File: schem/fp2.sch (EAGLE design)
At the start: 24 parts, among them IC1 74HC377N, IC10 74HC377N, IC11 74HC08N, IC12 ULN2003AN, IC13 ULN2003AN, IC14 ULN2003AN, IC15 74HC14N, IC2 74HC244N, IC3 74HC377N, IC4 74HC244N, IC5 74HC244N, IC6 74HC244N, IC7 74HC32N, IC8 74HC244N, IC9 74HC244N

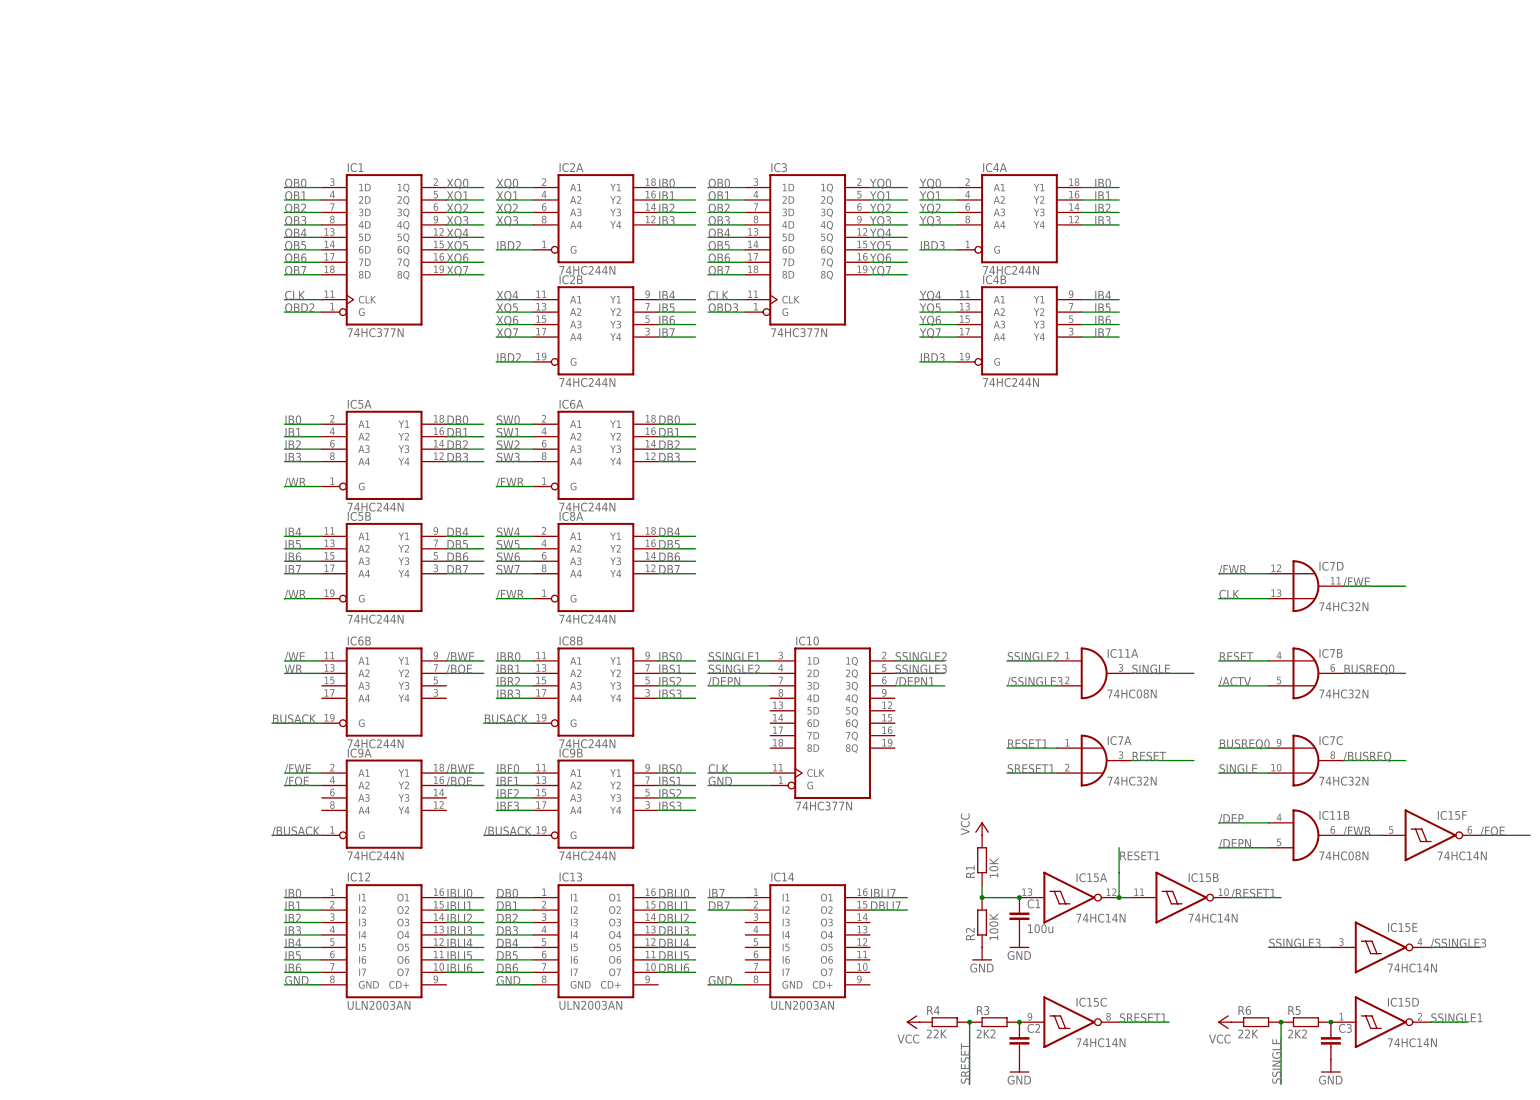
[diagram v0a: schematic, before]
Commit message: work on front panel boards
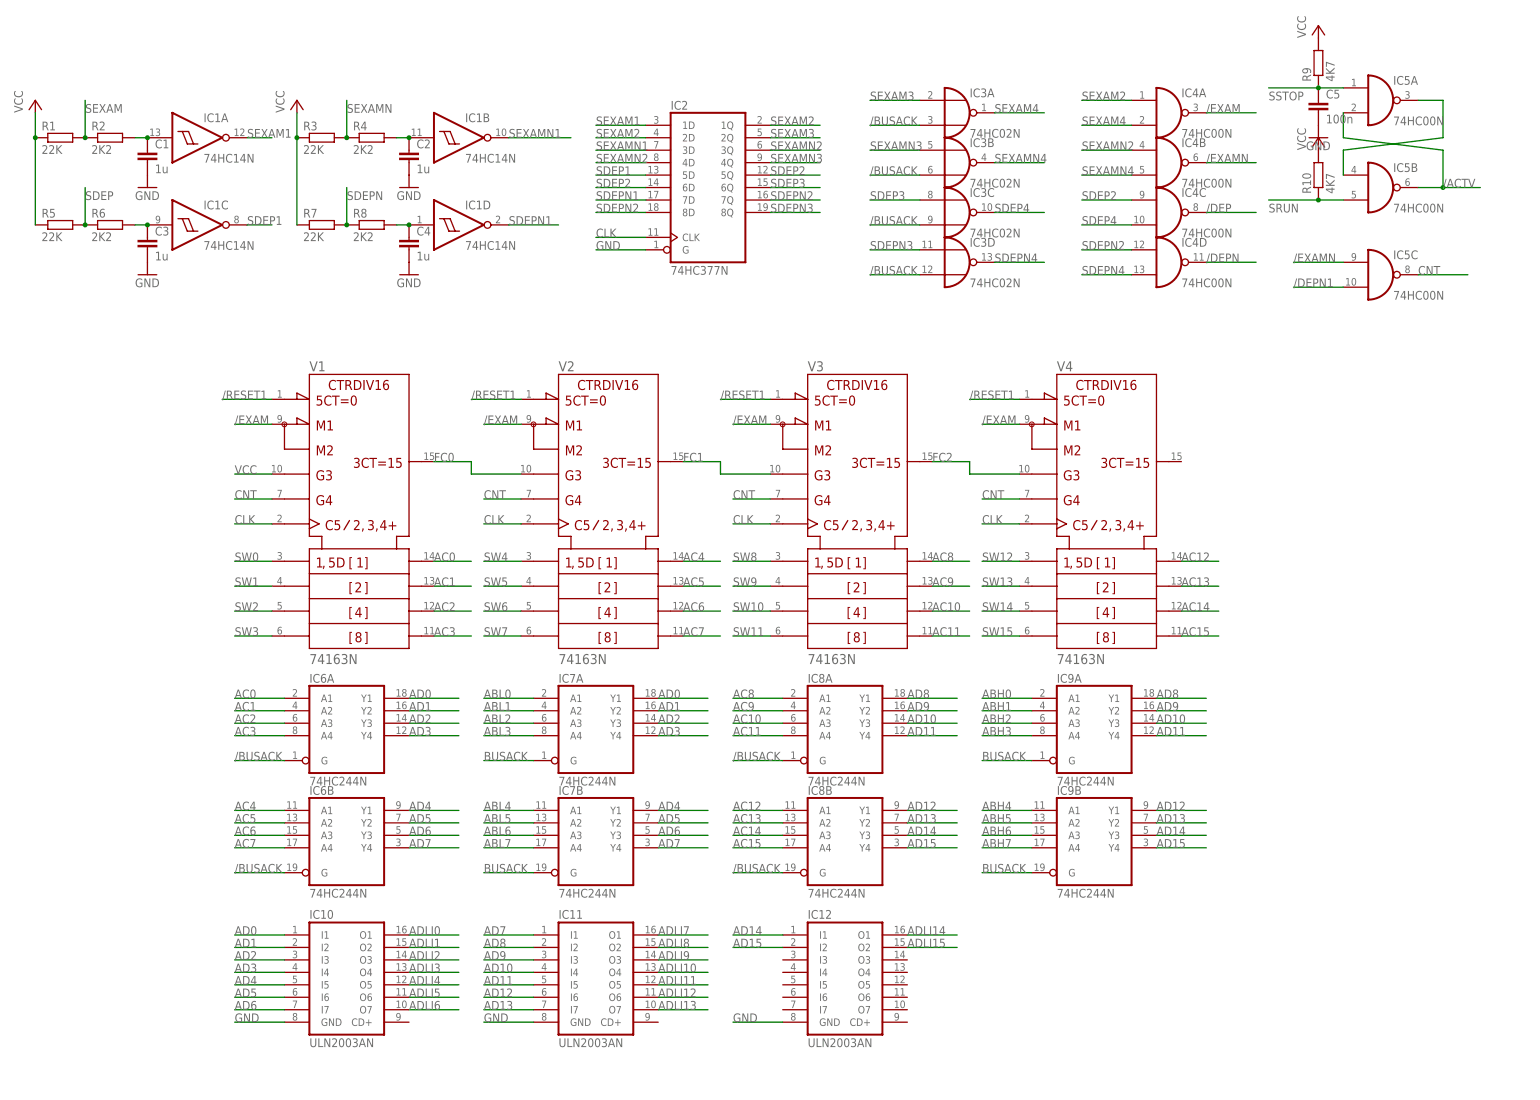
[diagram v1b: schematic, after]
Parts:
- removed IC13, IC14: ULN2003AN, uln-udn:ULN2003AN
- removed IC15: 74HC14N, 74xx-eu:74HC14N
- added C4: 1u, rcl:C-EU025-024X044
- added C5: 100n, rcl:C-EU025-024X044
- added R10, R9: 4K7, rcl:R-EU_0204/7
- added R7: 22K, rcl:R-EU_0204/7
- added R8: 2K2, rcl:R-EU_0204/7
- added V1, V2, V3, V4: 74163N, 74ttl-din:74163N
- C1: value 100u -> 1u
- C2, C3: value (none) -> 1u
- IC1: value 74HC377N -> 74HC14N; device 74xx-eu:74HC377N -> 74xx-eu:74HC14N
- IC10: value 74HC377N -> ULN2003AN; device 74xx-eu:74HC377N -> uln-udn:ULN2003AN
- IC11: value 74HC08N -> ULN2003AN; device 74xx-eu:74HC08N -> uln-udn:ULN2003AN
- IC2: value 74HC244N -> 74HC377N; device 74xx-eu:74HC244N -> 74xx-eu:74HC377N
- IC3: value 74HC377N -> 74HC02N; device 74xx-eu:74HC377N -> 74xx-eu:74HC02N
- IC4, IC5: value 74HC244N -> 74HC00N; device 74xx-eu:74HC244N -> 74xx-eu:74HC00N
- IC7: value 74HC32N -> 74HC244N; device 74xx-eu:74HC32N -> 74xx-eu:74HC244N
- R1: value 10K -> 22K; device rcl:R-EU_0207/7 -> rcl:R-EU_0204/7
- R2: value 100K -> 2K2; device rcl:R-EU_0207/7 -> rcl:R-EU_0204/7
- R3, R5: value 2K2 -> 22K; device rcl:R-EU_0207/7 -> rcl:R-EU_0204/7
- R4, R6: value 22K -> 2K2; device rcl:R-EU_0207/7 -> rcl:R-EU_0204/7
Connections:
- net IBF0 renamed ABH4
- net IBF1 renamed ABH5
- net IBF2 renamed ABH6
- net IBF3 renamed ABH7
- net IBLI0 renamed ADLI14
- net IBLI1 renamed ADLI15
- removed net /BOE: IC6B.Y2, IC9A.Y2
- removed net /BUSREQ: IC7C.O
- removed net /BWE: IC6B.Y1, IC9A.Y1
- removed net /FOE: IC15F.O, IC9A.A2
- removed net /FWE: IC7D.O, IC9A.A1
- removed net /FWR: IC11B.O, IC15F.I, IC6A.G, IC7D.I0, IC8A.G
- removed net /SSINGLE3: IC11A.I1, IC15E.O
- removed net /WE: IC6B.A1
- removed net /WR: IC5A.G, IC5B.G
- removed net BUSREQ0: IC7B.O, IC7C.I0
- removed net DB0: IC13.I1, IC5A.Y1, IC6A.Y1
- removed net DB1: IC13.I2, IC5A.Y2, IC6A.Y2
- removed net DB2: IC13.I3, IC5A.Y3, IC6A.Y3
- removed net DB3: IC13.I4, IC5A.Y4, IC6A.Y4
- removed net DB4: IC13.I5, IC5B.Y1, IC8A.Y1
- removed net DB5: IC13.I6, IC5B.Y2, IC8A.Y2
- removed net DB6: IC13.I7, IC5B.Y3, IC8A.Y3
- removed net DB7: IC14.I2, IC5B.Y4, IC8A.Y4
- removed net DBLI0: IC13.O1
- removed net DBLI1: IC13.O2
- removed net DBLI2: IC13.O3
- removed net DBLI3: IC13.O4
- removed net DBLI4: IC13.O5
- removed net DBLI5: IC13.O6
- removed net DBLI6: IC13.O7
- removed net DBLI7: IC14.O2
- removed net IB0: IC12.I1, IC2A.Y1, IC4A.Y1, IC5A.A1
- removed net IB1: IC12.I2, IC2A.Y2, IC4A.Y2, IC5A.A2
- removed net IB2: IC12.I3, IC2A.Y3, IC4A.Y3, IC5A.A3
- removed net IB3: IC12.I4, IC2A.Y4, IC4A.Y4, IC5A.A4
- removed net IB4: IC12.I5, IC2B.Y1, IC4B.Y1, IC5B.A1
- removed net IB5: IC12.I6, IC2B.Y2, IC4B.Y2, IC5B.A2
- removed net IB6: IC12.I7, IC2B.Y3, IC4B.Y3, IC5B.A3
- removed net IB7: IC14.I1, IC2B.Y4, IC4B.Y4, IC5B.A4
- removed net IBD2: IC2A.G, IC2B.G
- removed net IBD3: IC4A.G, IC4B.G
- removed net IBLI2: IC12.O3
- removed net IBLI3: IC12.O4
- removed net IBLI4: IC12.O5
- removed net IBLI5: IC12.O6
- removed net IBLI6: IC12.O7
- removed net IBLI7: IC14.O1
- removed net IBR0: IC8B.A1
- removed net IBR1: IC8B.A2
- removed net IBR2: IC8B.A3
- removed net IBR3: IC8B.A4
- removed net IBS0: IC8B.Y1, IC9B.Y1
- removed net IBS1: IC8B.Y2, IC9B.Y2
- removed net IBS2: IC8B.Y3, IC9B.Y3
- removed net IBS3: IC8B.Y4, IC9B.Y4
- removed net OB0: IC1A.1D, IC3A.1D
- removed net OB1: IC1A.2D, IC3A.2D
- removed net OB2: IC1A.3D, IC3A.3D
- removed net OB3: IC1A.4D, IC3A.4D
- removed net OB4: IC1A.5D, IC3A.5D
- removed net OB5: IC1A.6D, IC3A.6D
- removed net OB6: IC1A.7D, IC3A.7D
- removed net OB7: IC1A.8D, IC3A.8D
- removed net OBD2: IC1A.G
- removed net OBD3: IC3A.G
- removed net RESET: IC7A.O, IC7B.I0
- removed net RESET0: C1.1, IC15A.I, R1.1, R2.2
- removed net RESET1: IC15A.O, IC15B.I, IC7A.I0
- removed net SINGLE: IC11A.O, IC7C.I1
- removed net SRESET: R3.1, R4.2
- removed net SRESET0: C2.1, IC15C.I, R3.2
- removed net SRESET1: IC15C.O, IC7A.I1
- removed net SSINGLE: R5.1, R6.2
- removed net SSINGLE0: C3.1, IC15D.I, R5.2
- removed net SSINGLE1: IC10A.1D, IC15D.O
- removed net SSINGLE2: IC10A.1Q, IC10A.2D, IC11A.I0
- removed net SSINGLE3: IC10A.2Q, IC15E.I
- removed net WR: IC6B.A2
- removed net XQ0: IC1A.1Q, IC2A.A1
- removed net XQ1: IC1A.2Q, IC2A.A2
- removed net XQ2: IC1A.3Q, IC2A.A3
- removed net XQ3: IC1A.4Q, IC2A.A4
- removed net XQ4: IC1A.5Q, IC2B.A1
- removed net XQ5: IC1A.6Q, IC2B.A2
- removed net XQ6: IC1A.7Q, IC2B.A3
- removed net XQ7: IC1A.8Q, IC2B.A4
- removed net YQ0: IC3A.1Q, IC4A.A1
- removed net YQ1: IC3A.2Q, IC4A.A2
- removed net YQ2: IC3A.3Q, IC4A.A3
- removed net YQ3: IC3A.4Q, IC4A.A4
- removed net YQ4: IC3A.5Q, IC4B.A1
- removed net YQ5: IC3A.6Q, IC4B.A2
- removed net YQ6: IC3A.7Q, IC4B.A3
- removed net YQ7: IC3A.8Q, IC4B.A4
- new net /EXAM: IC4A.O, V11.!LOAD, V21.!LOAD, V31.!LOAD, V41.!LOAD
- new net /EXAMN: IC4B.O, IC5C.I0
- new net ABH0: IC9A.A1
- new net ABH1: IC9A.A2
- new net ABH2: IC9A.A3
- new net ABH3: IC9A.A4
- new net ABL0: IC7A.A1
- new net ABL1: IC7A.A2
- new net ABL2: IC7A.A3
- new net ABL3: IC7A.A4
- new net ABL4: IC7B.A1
- new net ABL5: IC7B.A2
- new net ABL6: IC7B.A3
- new net ABL7: IC7B.A4
- new net AC0: IC6A.A1, V11.QA
- new net AC1: IC6A.A2, V11.QB
- new net AC10: IC8A.A3, V31.QC
- new net AC11: IC8A.A4, V31.QD
- new net AC12: IC8B.A1, V41.QA
- new net AC13: IC8B.A2, V41.QB
- new net AC14: IC8B.A3, V41.QC
- new net AC15: IC8B.A4, V41.QD
- new net AC2: IC6A.A3, V11.QC
- new net AC3: IC6A.A4, V11.QD
- new net AC4: IC6B.A1, V21.QA
- new net AC5: IC6B.A2, V21.QB
- new net AC6: IC6B.A3, V21.QC
- new net AC7: IC6B.A4, V21.QD
- new net AC8: IC8A.A1, V31.QA
- new net AC9: IC8A.A2, V31.QB
- new net ACTV: IC5A.O, IC5B.I0
- new net AD0: IC10.I1, IC6A.Y1, IC7A.Y1
- new net AD1: IC10.I2, IC6A.Y2, IC7A.Y2
- new net AD10: IC11.I4, IC8A.Y3, IC9A.Y3
- new net AD11: IC11.I5, IC8A.Y4, IC9A.Y4
- new net AD12: IC11.I6, IC8B.Y1, IC9B.Y1
- new net AD13: IC11.I7, IC8B.Y2, IC9B.Y2
- new net AD14: IC12.I1, IC8B.Y3, IC9B.Y3
- new net AD15: IC12.I2, IC8B.Y4, IC9B.Y4
- new net AD2: IC10.I3, IC6A.Y3, IC7A.Y3
- new net AD3: IC10.I4, IC6A.Y4, IC7A.Y4
- new net AD4: IC10.I5, IC6B.Y1, IC7B.Y1
- new net AD5: IC10.I6, IC6B.Y2, IC7B.Y2
- new net AD6: IC10.I7, IC6B.Y3, IC7B.Y3
- new net AD7: IC11.I1, IC6B.Y4, IC7B.Y4
- new net AD8: IC11.I2, IC8A.Y1, IC9A.Y1
- new net AD9: IC11.I3, IC8A.Y2, IC9A.Y2
- new net ADLI0: IC10.O1
- new net ADLI1: IC10.O2
- new net ADLI10: IC11.O4
- new net ADLI11: IC11.O5
- new net ADLI12: IC11.O6
- new net ADLI13: IC11.O7
- new net ADLI2: IC10.O3
- new net ADLI3: IC10.O4
- new net ADLI4: IC10.O5
- new net ADLI5: IC10.O6
- new net ADLI6: IC10.O7
- new net ADLI7: IC11.O1
- new net ADLI8: IC11.O2
- new net ADLI9: IC11.O3
- new net CNT: IC5C.O, V11.ENP, V21.ENP, V31.ENP, V41.ENP
- new net FC0: V11.RCO, V21.ENT
- new net FC1: V21.RCO, V31.ENT
- new net FC2: V31.RCO, V41.ENT
- new net SDEP: R5.2, R6.1
- new net SDEP0: C3.1, IC1C.I, R6.2
- new net SDEP1: IC1C.O, IC2A.5D
- new net SDEP2: IC2A.5Q, IC2A.6D, IC4C.I0
- new net SDEP3: IC2A.6Q, IC3C.I0
- new net SDEP4: IC3C.O, IC4C.I1
- new net SDEPN: R7.2, R8.1
- new net SDEPN0: C4.1, IC1D.I, R8.2
- new net SDEPN1: IC1D.O, IC2A.7D
- new net SDEPN2: IC2A.7Q, IC2A.8D, IC4D.I0
- new net SDEPN3: IC2A.8Q, IC3D.I0
- new net SDEPN4: IC3D.O, IC4D.I1
- new net SEXAM: R1.2, R2.1
- new net SEXAM0: C1.1, IC1A.I, R2.2
- new net SEXAM1: IC1A.O, IC2A.1D
- new net SEXAM2: IC2A.1Q, IC2A.2D, IC4A.I0
- new net SEXAM3: IC2A.2Q, IC3A.I0
- new net SEXAM4: IC3A.O, IC4A.I1
- new net SEXAMN: R3.2, R4.1
- new net SEXAMN0: C2.1, IC1B.I, R4.2
- new net SEXAMN1: IC1B.O, IC2A.3D
- new net SEXAMN2: IC2A.3Q, IC2A.4D, IC4B.I0
- new net SEXAMN3: IC2A.4Q, IC3B.I0
- new net SEXAMN4: IC3B.O, IC4B.I1
- new net SRUN: IC5B.I1, R10.1
- new net SSTOP: C5.1, IC5A.I0, R9.1
- new net SW10: V31.C
- new net SW11: V31.D
- new net SW12: V41.A
- new net SW13: V41.B
- new net SW14: V41.C
- new net SW15: V41.D
- new net SW8: V31.A
- new net SW9: V31.B
- net /ACTV: now also IC5A.I1, IC5B.O; no longer IC7B.I1
- net /BUSACK: now also IC3A.I1, IC3B.I1, IC3C.I1, IC3D.I1, IC6A.G, IC6B.G, IC8A.G, IC8B.G; no longer IC9A.G, IC9B.G
- net /DEP: now also IC4C.O; no longer IC11B.I0
- net /DEPN: now also IC4D.O; no longer IC10A.3D, IC11B.I1
- net /DEPN1: now also IC5C.I1; no longer IC10A.3Q
- net /RESET1: now also V11.!CLR, V21.!CLR, V31.!CLR, V41.!CLR; no longer IC15B.O
- net BUSACK: now also IC7A.G, IC7B.G, IC9A.G, IC9B.G; no longer IC6B.G, IC8B.G
- net CLK: now also IC2A.CLK, V11.CLK, V21.CLK, V31.CLK, V41.CLK; no longer IC10A.CLK, IC1A.CLK, IC3A.CLK, IC7D.I1
- net GND: now also C4.2, C5.2, IC10.GND, IC11.GND, IC2A.G; no longer IC10A.G, IC13.GND, IC14.GND, R2.1
- net SW0: now also V11.A; no longer IC6A.A1
- net SW1: now also V11.B; no longer IC6A.A2
- net SW2: now also V11.C; no longer IC6A.A3
- net SW3: now also V11.D; no longer IC6A.A4
- net SW4: now also V21.A; no longer IC8A.A1
- net SW5: now also V21.B; no longer IC8A.A2
- net SW6: now also V21.C; no longer IC8A.A3
- net SW7: now also V21.D; no longer IC8A.A4
- net VCC: now also R1.1, R10.2, R3.1, R5.1, R7.1, R9.2, V11.ENT; no longer R1.2, R4.1, R6.1
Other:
- moved on the sheet: C1, C2, C3, IC12, IC6A, IC6B, IC8A, IC8B, IC9A, IC9B, R1, R2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
